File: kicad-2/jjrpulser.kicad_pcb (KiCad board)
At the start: 2 copper layers, 20 parts, among them J1 USB_OTG, J3 Screw_Terminal_HOT, J4 Screw_Terminal_COLD, J5 Conn_UART, U1 ESP-12, U2 NCP1117-3.3_SOT223

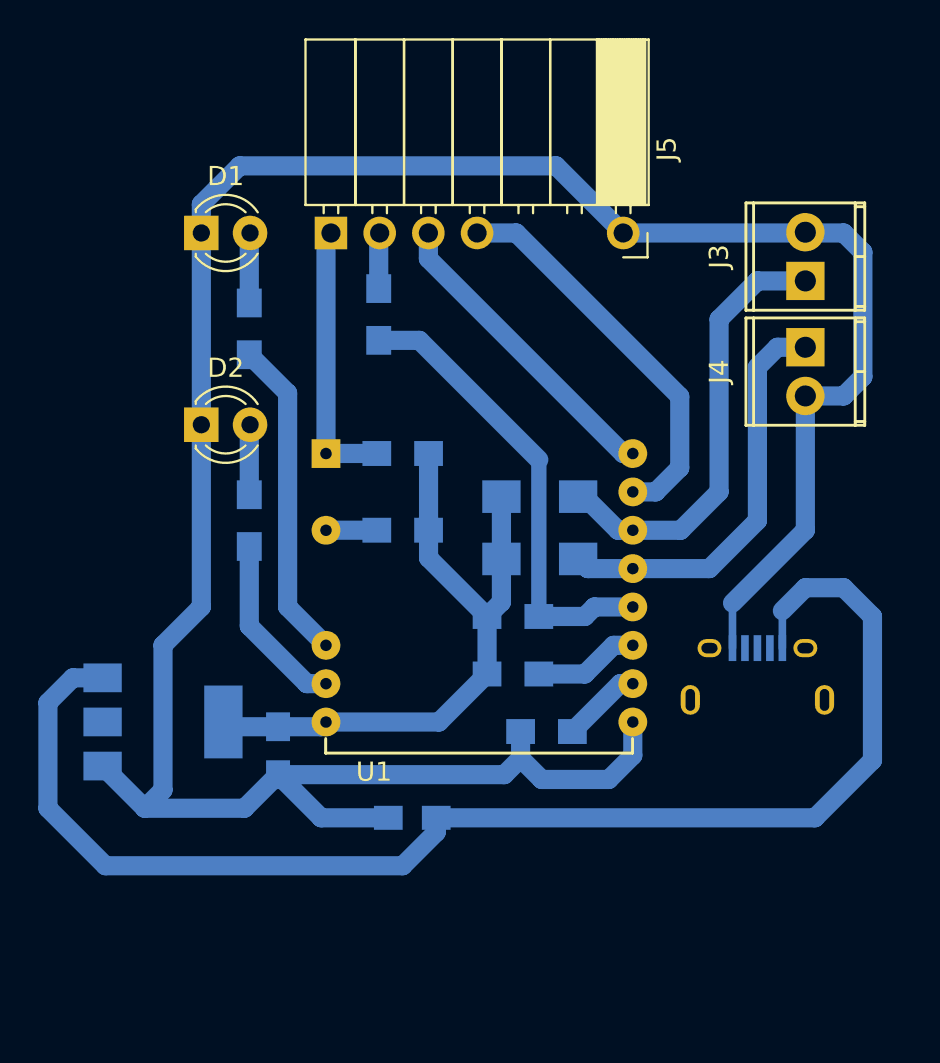
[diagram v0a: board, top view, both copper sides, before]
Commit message: Разводка в процессе
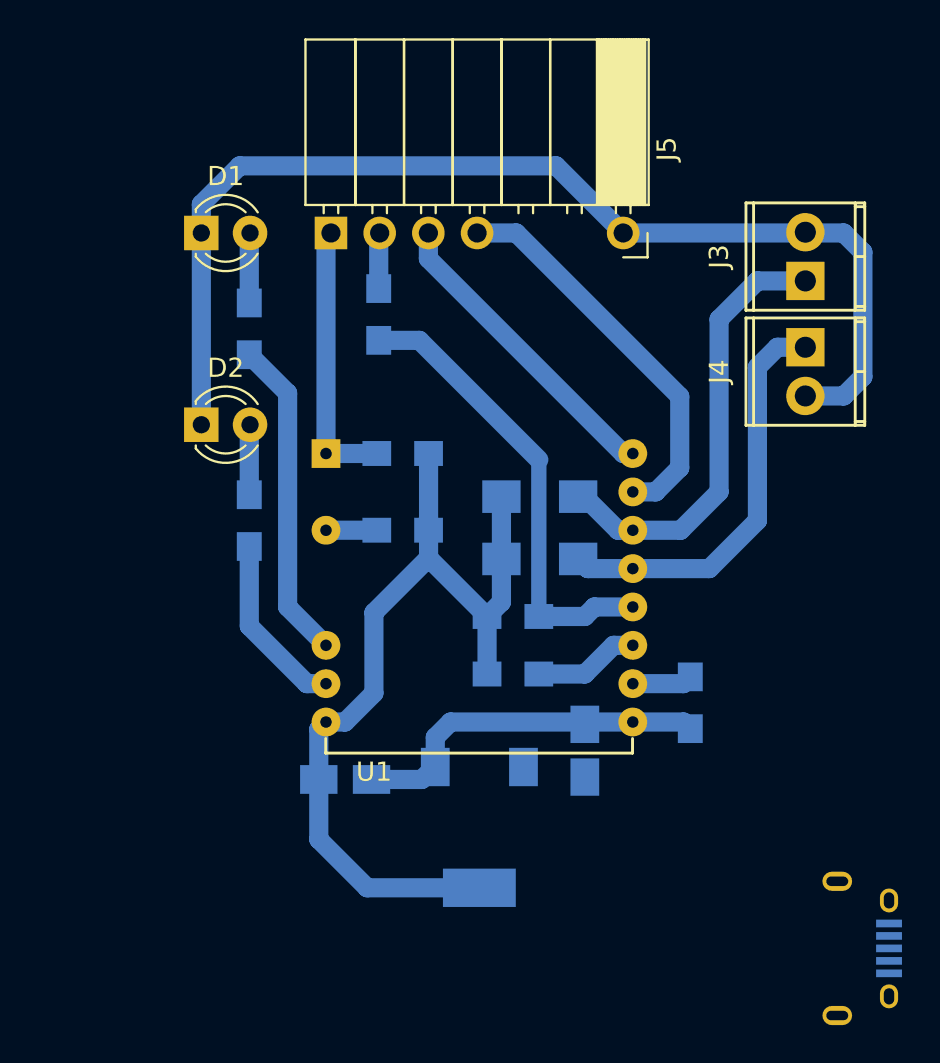
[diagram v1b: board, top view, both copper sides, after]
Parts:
- C1, C2: footprint Capacitors_SMD:C_0805_HandSoldering -> Capacitors_Tantalum_SMD:CP_Tantalum_Case-A_EIA-3216-18_Reflow
- moved U2 17.4 mm to (155.5, 124.5), turned to 270 degrees
- moved J1 15.3 mm to (175.5, 130.8), turned to 90 degrees
- moved C1 9.66 mm to (161.0, 120.5), turned to 90 degrees
- moved R6 7.65 mm to (166.5, 118.0), turned to 90 degrees
- moved C2 3.81 mm to (148.5, 122.0), turned to 0 degrees
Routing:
- net Net-(C1-Pad1): track 71.1 -> 0.00 mm
- net Earth: track 135.0 -> 77.5 mm
- net +3V3: track 34.3 -> 46.4 mm
- net Net-(R6-Pad2): track 4.19 -> 3.15 mm
